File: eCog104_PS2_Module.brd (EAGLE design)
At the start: 48 x 28 mm, 1 part

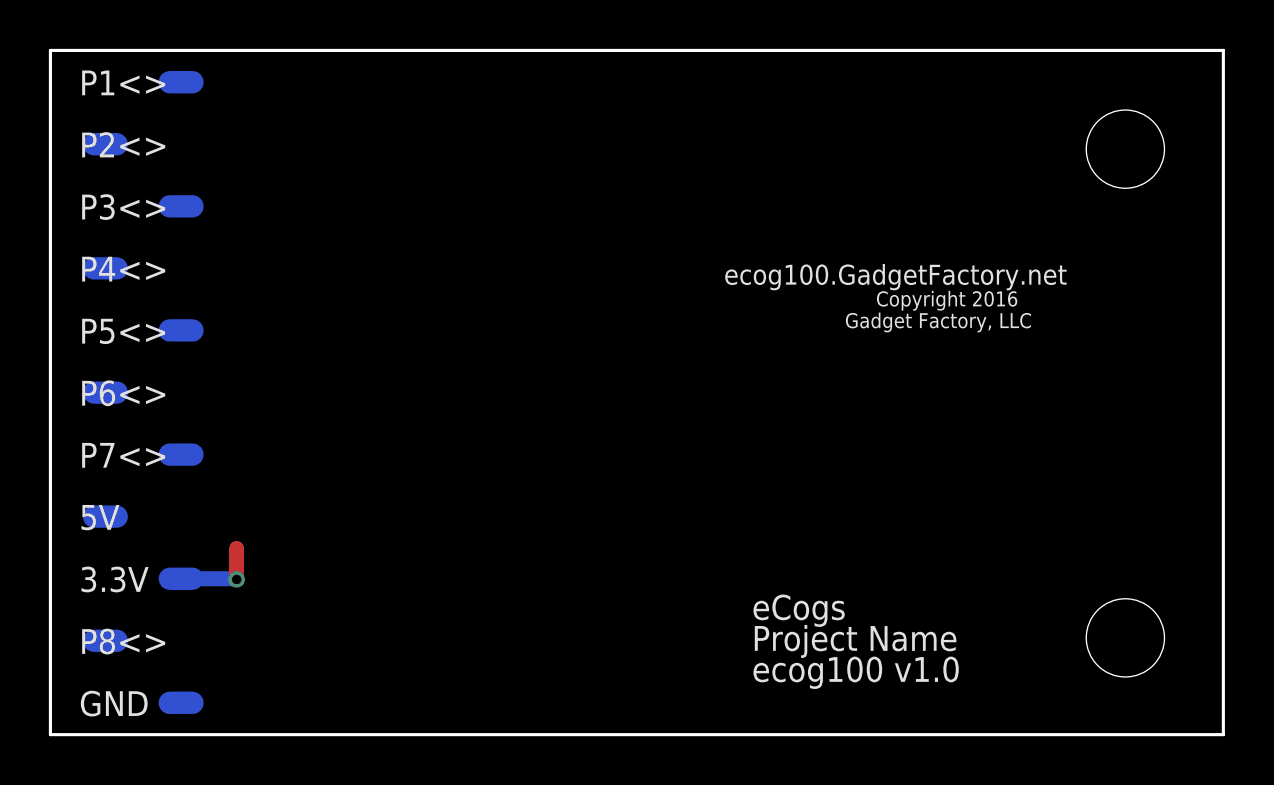
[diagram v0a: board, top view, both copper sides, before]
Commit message: V1.1
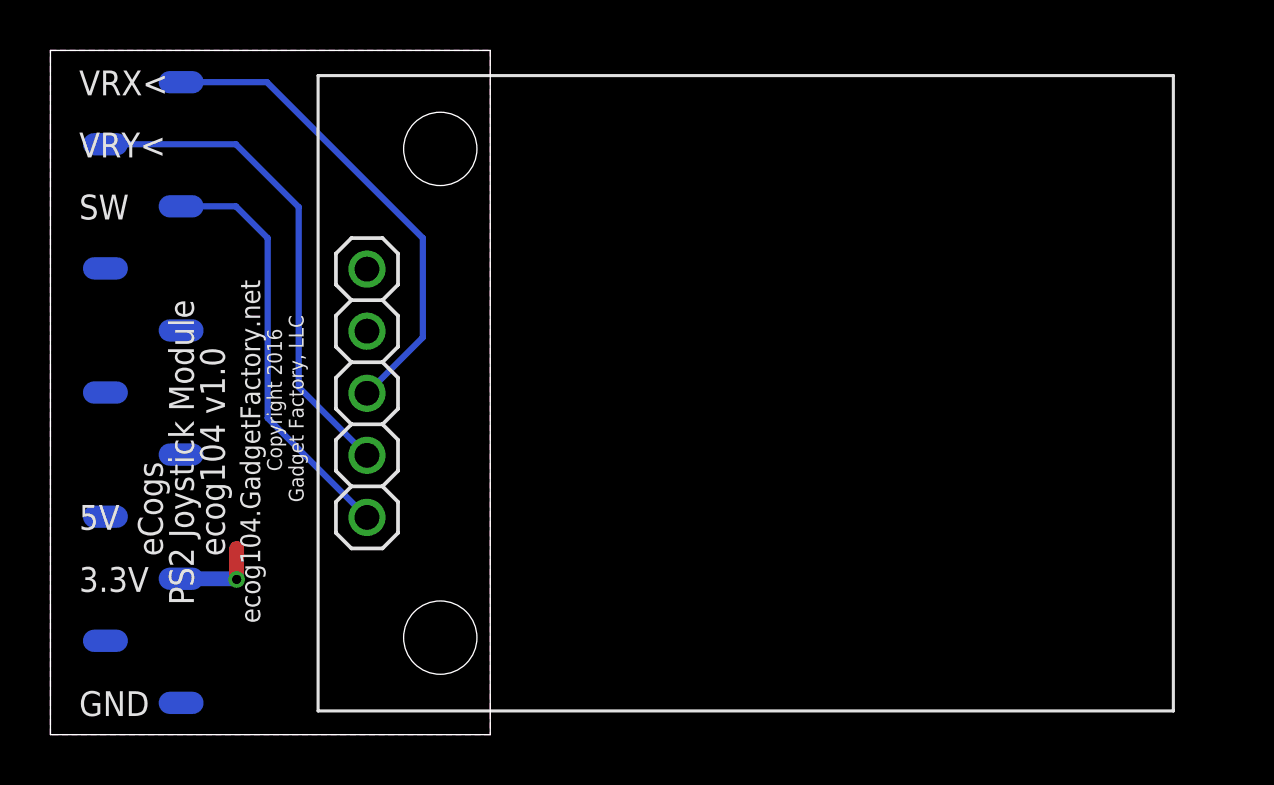
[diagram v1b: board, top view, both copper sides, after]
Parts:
- added JP1: (no value), eCogs:PS2-MODULE
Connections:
- new net A1: ECOG.1, JP1.VRX
- new net A2: ECOG.2, JP1.VRY
- new net A3: ECOG.3, JP1.SW
- net 3V3: now also JP1.VCC
- net GND: now also JP1.GND
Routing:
- net A2: track 0.00 -> 20.3 mm
- net A1: track 0.00 -> 19.8 mm
- net A3: track 0.00 -> 17.2 mm
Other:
- board size 48 x 28 mm -> 18 x 28 mm
- board text added: "PS2 Joystick Module"
- board text added: "SW"
- board text added: "VRX<"
- board text added: "VRY<"
- board text added: "ecog104 v1.0"
- board text added: "ecog104.GadgetFactory.net"
- board text removed: "P1<>"
- board text removed: "P2<>"
- board text removed: "P3<>"
- board text removed: "P4<>"
- board text removed: "P5<>"
- board text removed: "P6<>"
- board text removed: "P7<>"
- board text removed: "P8<>"
- board text removed: "Project Name"
- board text removed: "ecog100 v1.0"
- board text removed: "ecog100.GadgetFactory.net"
